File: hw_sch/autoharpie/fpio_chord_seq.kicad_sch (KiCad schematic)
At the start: 144 parts, among them SW10 SW_Push_45deg, SW11 SW_Push_45deg, SW12 SW_Push_45deg, SW13 SW_Push_45deg, SW14 SW_Push_45deg, SW15 SW_Push_45deg, SW16 SW_Push_45deg, SW17 SW_Push_45deg, SW18 SW_Push_45deg, SW19 SW_Push_45deg, SW20 SW_Push_45deg, SW21 SW_Push_45deg, SW22 SW_Push_45deg, SW23 SW_Push_45deg, SW24 SW_Push_45deg, SW25 SW_Push_45deg, SW26 SW_Push_45deg, SW27 SW_Push_45deg, SW28 SW_Push_45deg, SW29 SW_Push_45deg, SW30 SW_Push_45deg, SW31 SW_Push_45deg, SW32 SW_Push_45deg, SW33 SW_Push_45deg, SW34 SW_Push_45deg, SW35 SW_Push_45deg, SW36 SW_Push_45deg, SW37 SW_Push_45deg, SW38 SW_Push_45deg, SW39 SW_Push_45deg, SW4 SW_Push_45deg, SW40 SW_Push_45deg, SW41 SW_Push_45deg, SW42 SW_Push_45deg, SW43 SW_Push_45deg, SW44 SW_Push_45deg, SW45 SW_Push_45deg, SW46 SW_Push_45deg, SW47 SW_Push_45deg, SW48 SW_Push_45deg, SW49 SW_Push_45deg, SW5 SW_Push_45deg, SW50 SW_Push_45deg, SW51 SW_Push_45deg, SW52 SW_Push_45deg, SW53 SW_Push_45deg, SW54 SW_Push_45deg, SW55 SW_Push_45deg, SW56 SW_Push_45deg, SW57 SW_Push_45deg, SW58 SW_Push_45deg, SW59 SW_Push_45deg, SW6 SW_Push_45deg, SW60 SW_Push_45deg, SW61 SW_Push_45deg, SW62 SW_Push_45deg, SW63 SW_Push_45deg, SW64 SW_Push_45deg, SW65 SW_Push_45deg, SW66 SW_Push_45deg, SW67 SW_Push_45deg, SW68 SW_Push_45deg, SW69 SW_Push_45deg, SW7 SW_Push_45deg, SW70 SW_Push_45deg, SW71 SW_Push_45deg, SW72 SW_Push_45deg, SW73 SW_Push_45deg, SW74 SW_Push_45deg, SW75 SW_Push_45deg, SW8 SW_Push_45deg, SW9 SW_Push_45deg

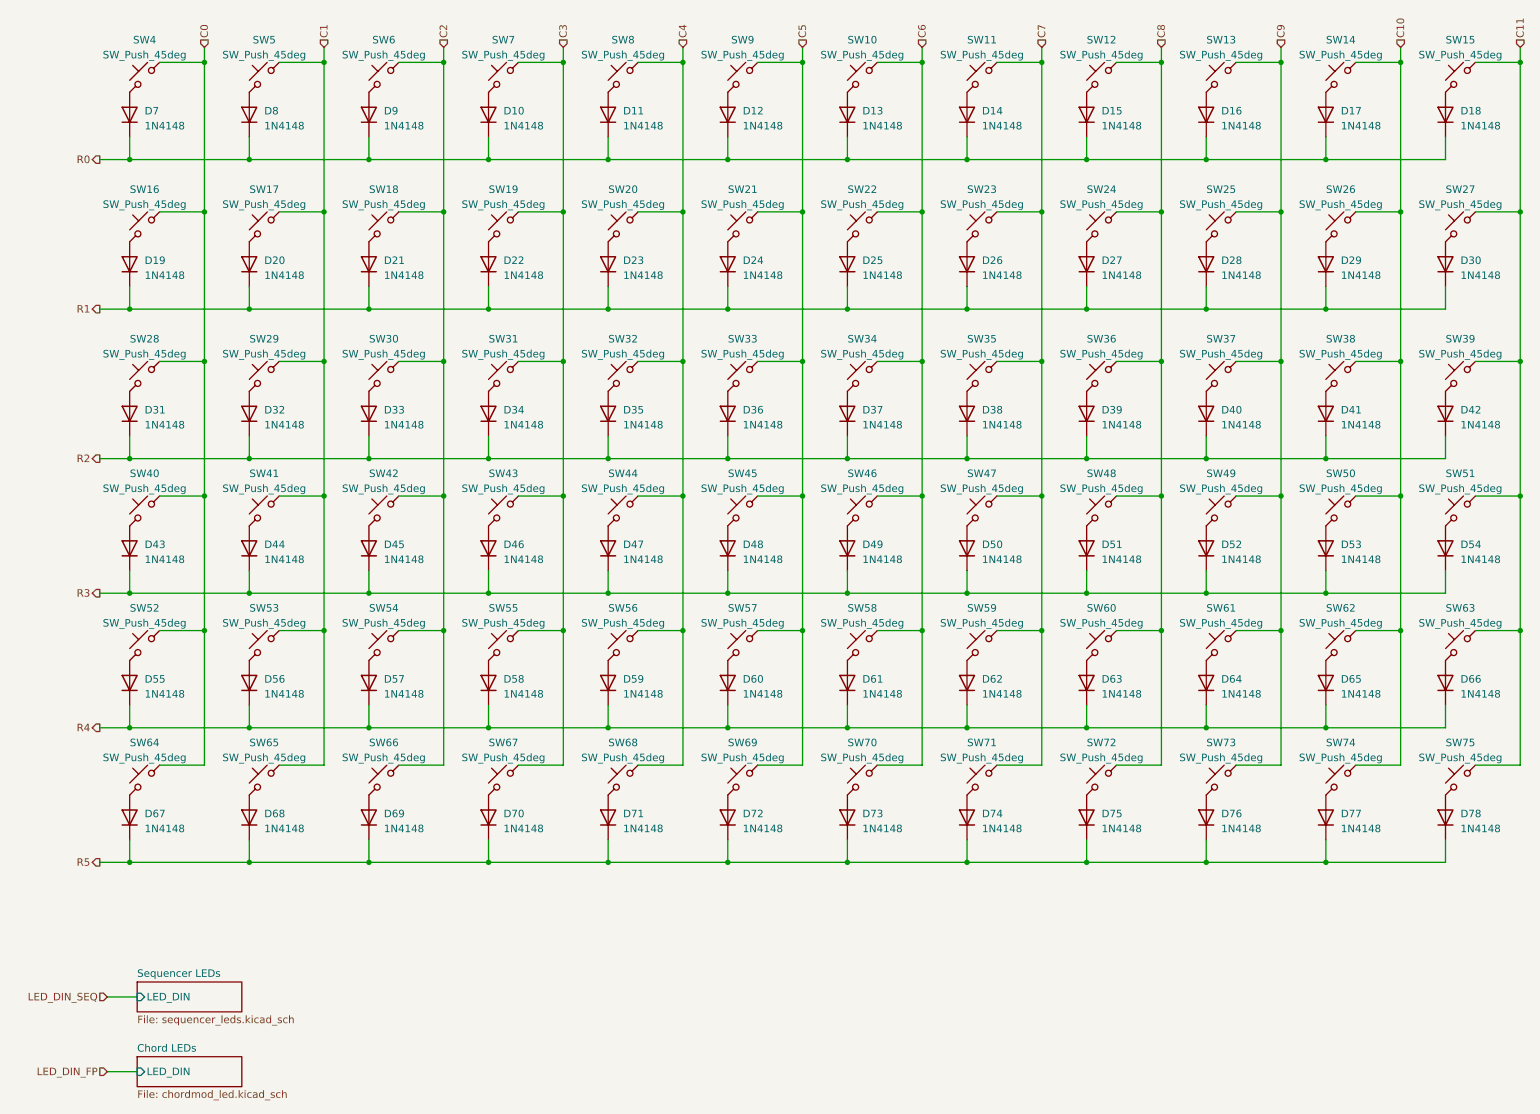
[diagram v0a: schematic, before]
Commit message: rev 0.1 pcb
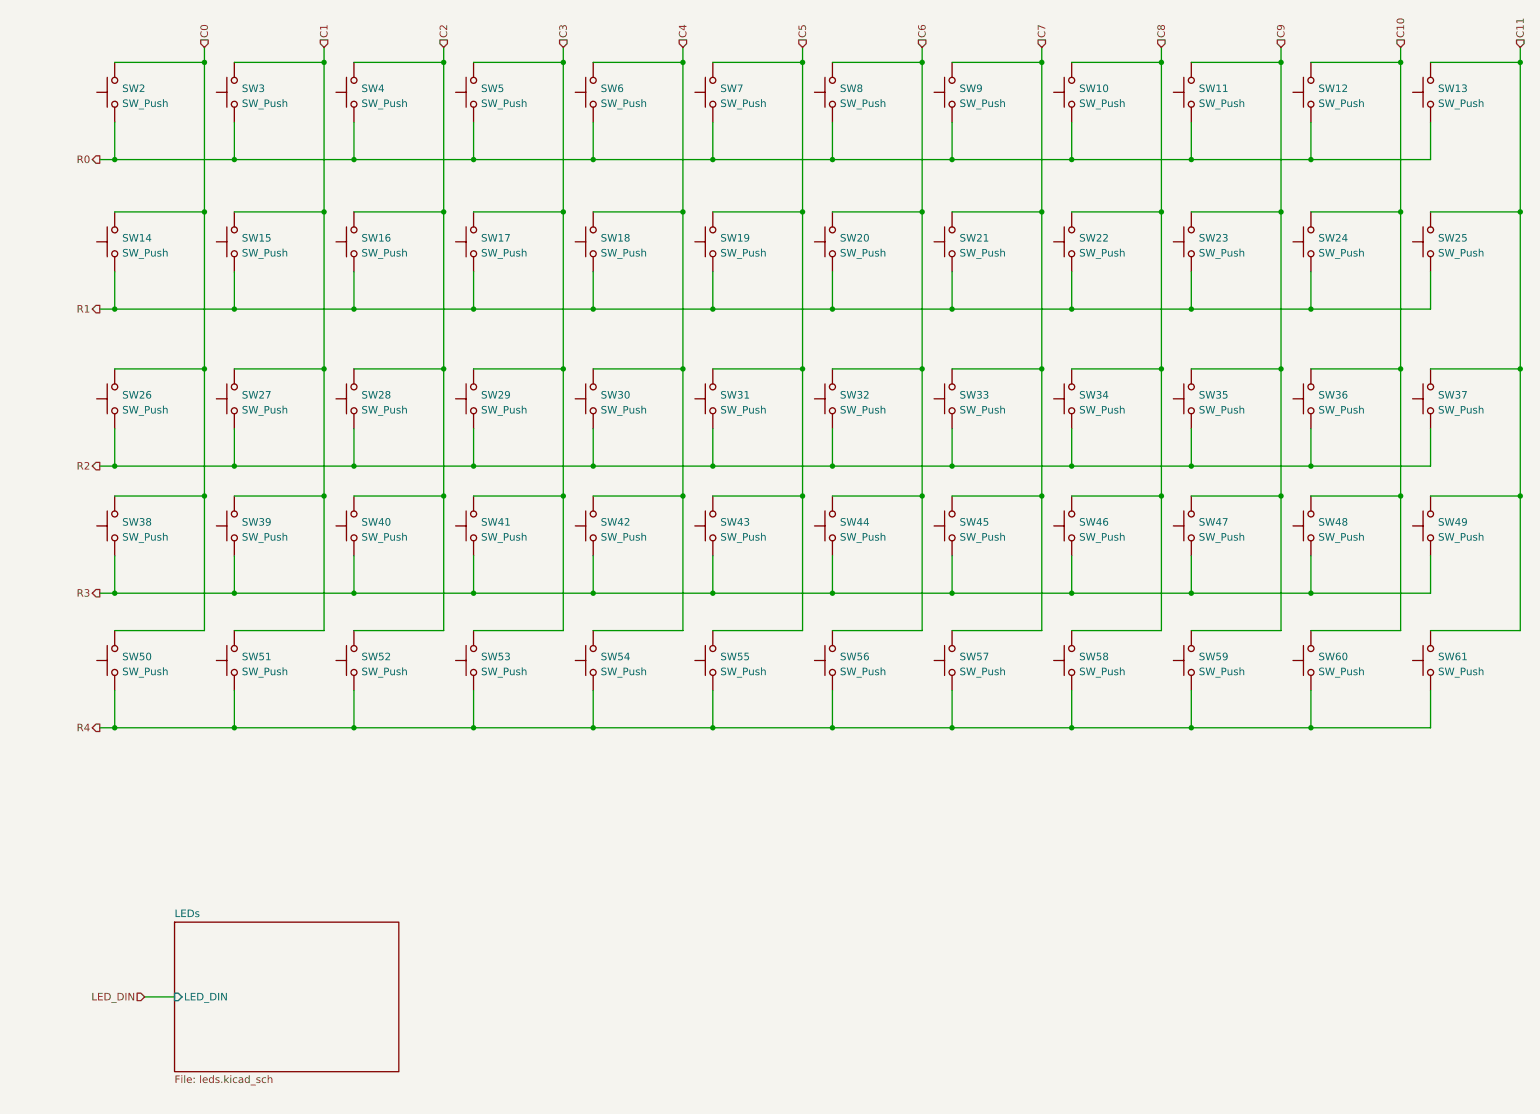
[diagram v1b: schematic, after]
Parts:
- removed D10, D11, D12, D13, D14, D15, D16, D17, D18, D19, D20, D21, D22, D23, D24, D25, D26, D27, D28, D29, D30, D31, D32, D33, D34, D35, D36, D37, D38, D39, D40, D41, D42, D43, D44, D45, D46, D47, D48, D49, D50, D51, D52, D53, D54, D55, D56, D57, D58, D59, D60, D61, D62, D63, D64, D65, D66, D67, D68, D69, D7, D70, D71, D72, D73, D74, D75, D76, D77, D78, D8, D9: 1N4148, Diode_THT:D_DO-35_SOD27_P7.62mm_Horizontal, symbol Device:D
- removed SW10, SW11, SW12, SW13, SW14, SW15, SW16, SW17, SW18, SW19, SW20, SW21, SW22, SW23, SW24, SW25, SW26, SW27, SW28, SW29, SW30, SW31, SW32, SW33, SW34, SW35, SW36, SW37, SW38, SW39, SW4, SW40, SW41, SW42, SW43, SW44, SW45, SW46, SW47, SW48, SW49, SW5, SW50, SW51, SW52, SW53, SW54, SW55, SW56, SW57, SW58, SW59, SW6, SW60, SW61, SW62, SW63, SW64, SW65, SW66, SW67, SW68, SW69, SW7, SW70, SW71, SW72, SW73, SW74, SW75, SW8, SW9: SW_Push_45deg, Button_Switch_THT:SW_PUSH_6mm_H4.3mm, symbol Switch:SW_Push_45deg
- added SW10, SW11, SW12, SW13, SW14, SW15, SW16, SW17, SW18, SW19, SW2, SW20, SW21, SW22, SW23, SW24, SW25, SW26, SW27, SW28, SW29, SW3, SW30, SW31, SW32, SW33, SW34, SW35, SW36, SW37, SW38, SW39, SW4, SW40, SW41, SW42, SW43, SW44, SW45, SW46, SW47, SW48, SW49, SW5, SW50, SW51, SW52, SW53, SW54, SW55, SW56, SW57, SW58, SW59, SW6, SW60, SW61, SW7, SW8, SW9: SW_Push, Button_Switch_THT:SW_PUSH_6mm, symbol Switch:SW_Push
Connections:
- net C0: now also SW14.2, SW2.2, SW26.2, SW38.2, SW50.2
- net C1: now also SW15.2, SW27.2, SW3.2, SW39.2, SW51.2
- net C10: now also SW12.2, SW24.2, SW36.2, SW48.2, SW60.2
- net C11: now also SW13.2, SW25.2, SW37.2, SW49.2, SW61.2
- net C2: now also SW16.2, SW28.2, SW4.2, SW40.2, SW52.2
- net C3: now also SW17.2, SW29.2, SW41.2, SW5.2, SW53.2
- net C4: now also SW18.2, SW30.2, SW42.2, SW54.2, SW6.2
- net C5: now also SW19.2, SW31.2, SW43.2, SW55.2, SW7.2
- net C6: now also SW20.2, SW32.2, SW44.2, SW56.2, SW8.2
- net C7: now also SW21.2, SW33.2, SW45.2, SW57.2, SW9.2
- net C8: now also SW10.2, SW22.2, SW34.2, SW46.2, SW58.2
- net C9: now also SW11.2, SW23.2, SW35.2, SW47.2, SW59.2
- net R0: now also SW10.1, SW11.1, SW12.1, SW13.1, SW2.1, SW3.1, SW4.1, SW5.1, SW6.1, SW7.1, SW8.1, SW9.1
- net R1: now also SW14.1, SW15.1, SW16.1, SW17.1, SW18.1, SW19.1, SW20.1, SW21.1, SW22.1, SW23.1, SW24.1, SW25.1
- net R2: now also SW26.1, SW27.1, SW28.1, SW29.1, SW30.1, SW31.1, SW32.1, SW33.1, SW34.1, SW35.1, SW36.1, SW37.1
- net R3: now also SW38.1, SW39.1, SW40.1, SW41.1, SW42.1, SW43.1, SW44.1, SW45.1, SW46.1, SW47.1, SW48.1, SW49.1
- net R4: now also SW50.1, SW51.1, SW52.1, SW53.1, SW54.1, SW55.1, SW56.1, SW57.1, SW58.1, SW59.1, SW60.1, SW61.1
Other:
- removed sheet Chord LEDs
- removed sheet Sequencer LEDs
- added sheet LEDs (leds.kicad_sch)
